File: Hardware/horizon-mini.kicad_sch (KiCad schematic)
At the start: 77 parts, among them J2 Conn_01x02_Pin, J3 Micro_SD_Card_Det1, J7 USB_C_Receptacle_USB2.0_16P, J8 Conn_02x03_Counter_Clockwise, Q1 BSS138, Q10 DMG2301L, U1 TPS82130, U16 AP2112K-3.3, U2 TPS61092, U3 LTC4412xS6, U5 ATSAMD21G18A-A, U6 NAND, U7 LPS22HB, U9 LSM6DS3

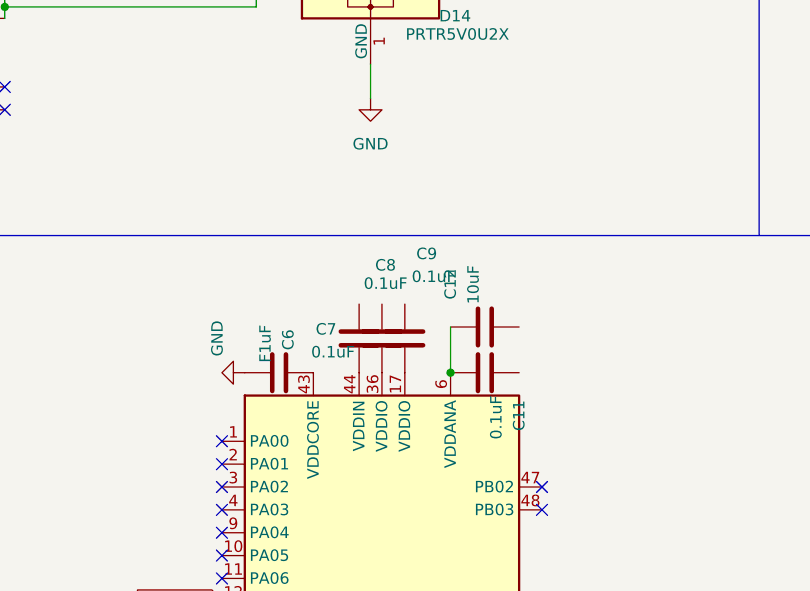
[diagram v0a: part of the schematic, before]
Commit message: fixed schematic
i hate github
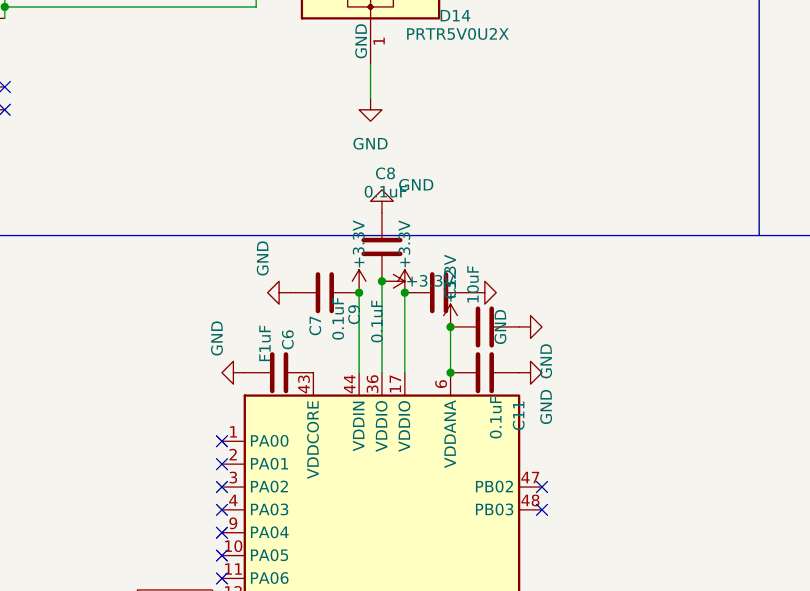
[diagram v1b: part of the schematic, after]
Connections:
- net +3.3V: now also C11.2, C12.1, C7.2, C8.2, C9.1, U5.17 (VDDIO), U5.36 (VDDIO), U5.44 (VDDIN), U5.6 (VDDANA)
- net GND: now also C11.1, C12.2, C7.1, C8.1, C9.2
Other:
- moved on the sheet: C7, C8, C9
